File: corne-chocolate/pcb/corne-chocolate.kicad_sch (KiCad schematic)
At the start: 87 parts, among them J1 MJ-4PP-9, J2 OLED, J3 LED, P1 i2c-pin, P2 i2c-pin, SW1 SW_PUSH, SW10 SW_PUSH, SW11 SW_PUSH, SW12 SW_PUSH, SW13 SW_PUSH, SW14 SW_PUSH, SW15 SW_PUSH, SW16 SW_PUSH, SW17 SW_PUSH, SW18 SW_PUSH, SW19 SW_PUSH, SW2 SW_PUSH, SW20 SW_PUSH, SW21 SW_PUSH, SW3 SW_PUSH, SW4 SW_PUSH, SW5 SW_PUSH, SW6 SW_PUSH, SW7 SW_PUSH, SW8 SW_PUSH, SW9 SW_PUSH, U1 ProMicro

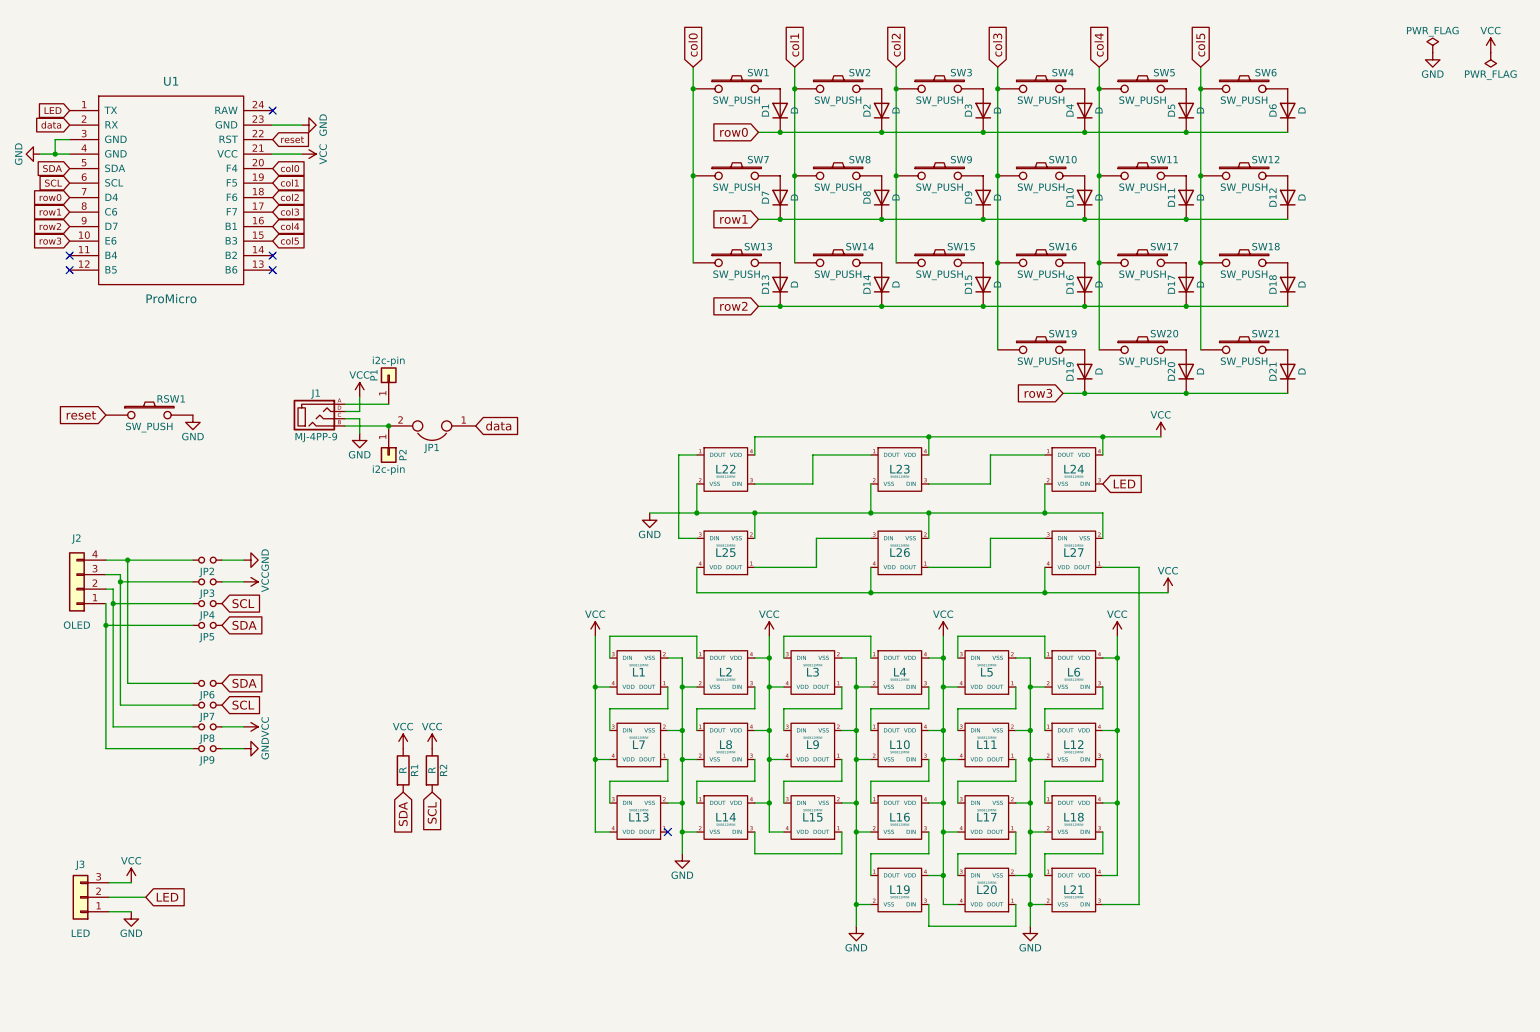
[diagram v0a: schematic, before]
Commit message: Cleanup schematic
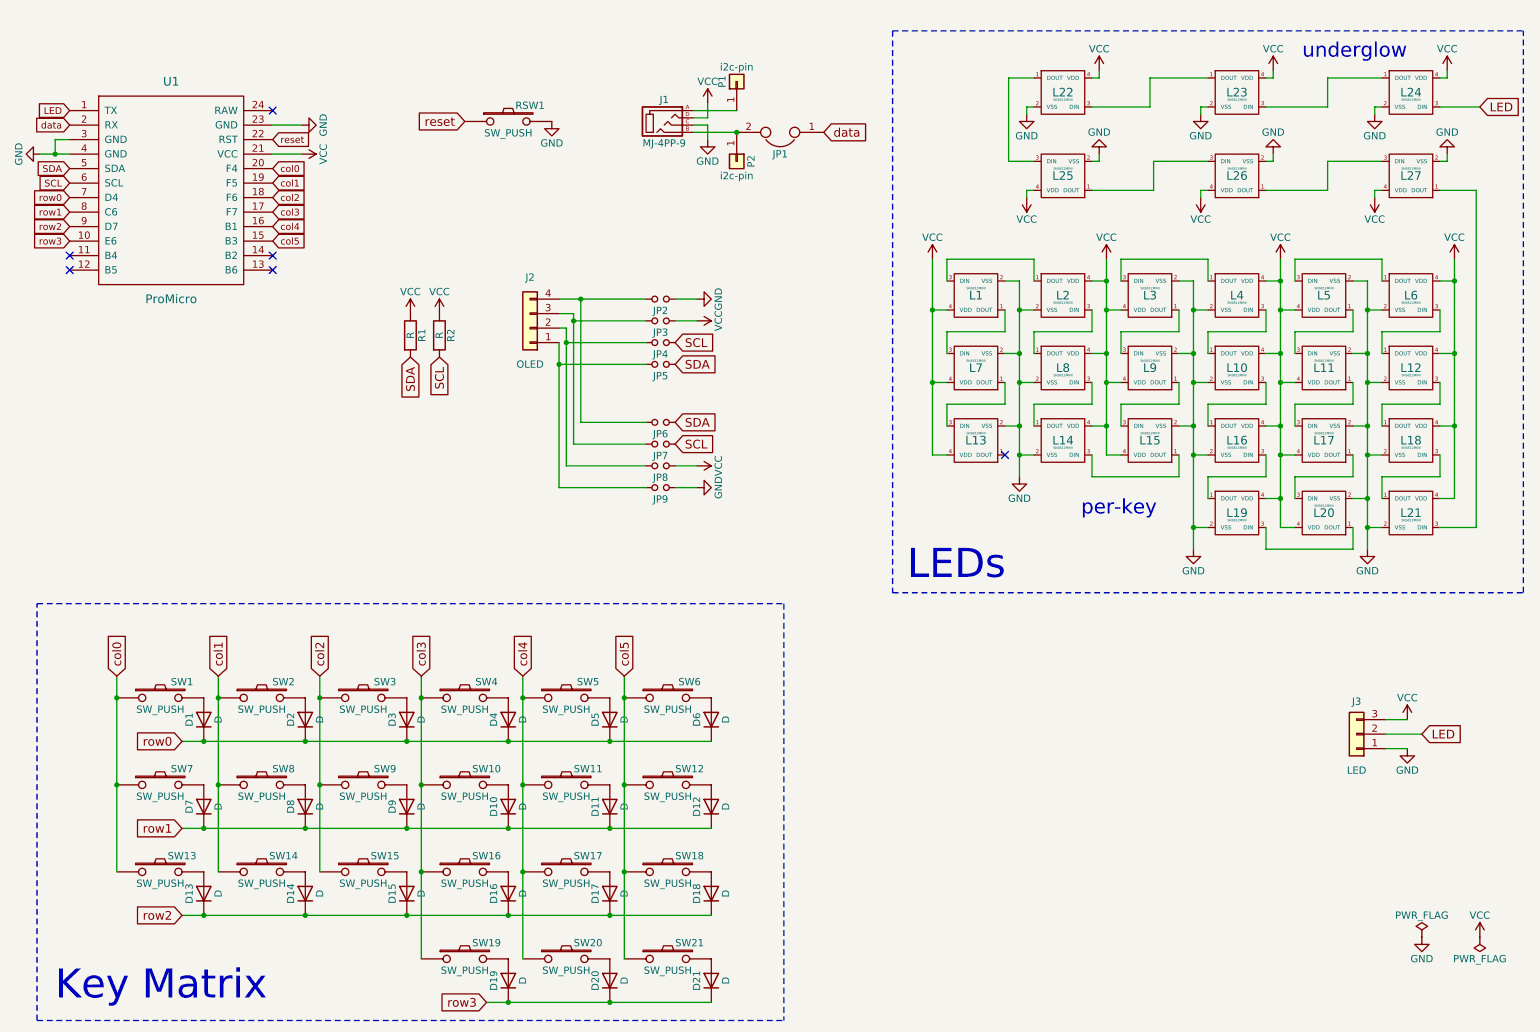
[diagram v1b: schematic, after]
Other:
- note added: "Key Matrix"
- note added: "LEDs"
- note added: "per-key"
- note added: "underglow"
- moved on the sheet: D1, D10, D11, D12, D13, D14, D15, D16, D17, D18, D19, D2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
